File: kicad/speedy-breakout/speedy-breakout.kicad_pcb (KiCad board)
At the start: 2 copper layers, 100 x 50 mm, 7 parts, among them J1 Pin Socket 1x20, J2 Pin Socket 1x20, J3 Molex Mini-Lock 53426, J4 Molex Mini-Lock 53426, J5 CUI TLB009-254, J6 CUI TBL009-254

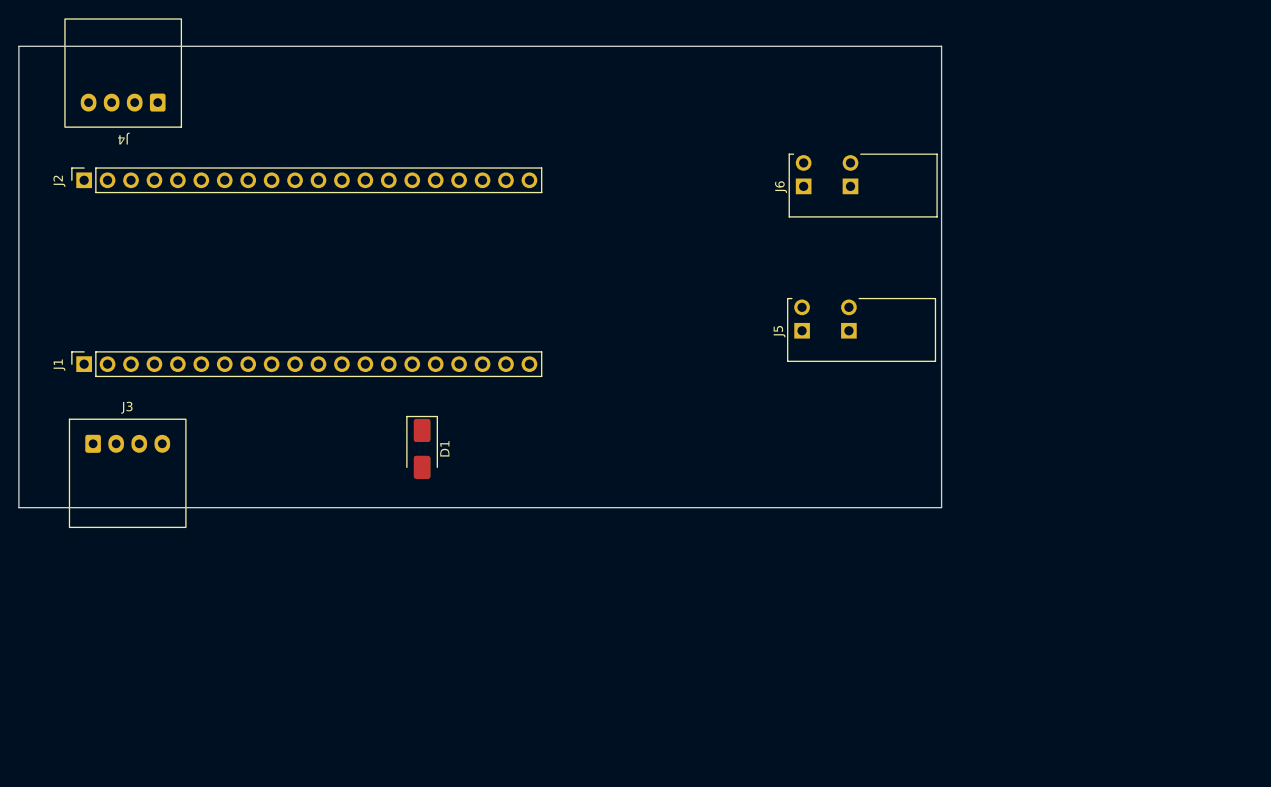
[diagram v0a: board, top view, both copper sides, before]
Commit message: speedy-breakout: Complete Rev 1.0 Schematics/Layout
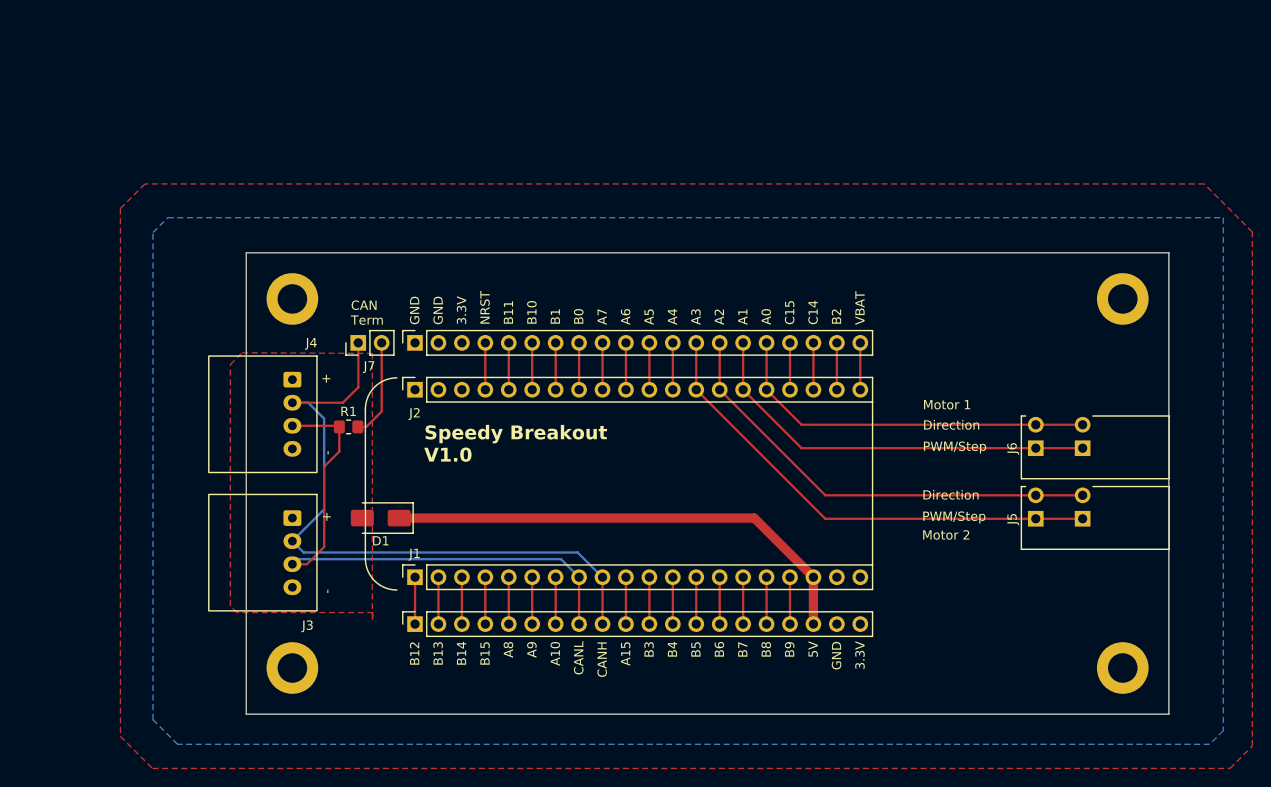
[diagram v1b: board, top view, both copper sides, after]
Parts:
- added ?: Pin Socket 1x20, Connector_PinSocket_2.54mm:PinSocket_1x20_P2.54mm_Vertical, F.Cu at (118.3, 84.8)
- added ?: Pin Socket 1x20, Connector_PinSocket_2.54mm:PinSocket_1x20_P2.54mm_Vertical, F.Cu at (118.3, 115.2)
- added J7: Conn_01x02, Connector_PinHeader_2.54mm:PinHeader_1x02_P2.54mm_Vertical, F.Cu at (112.1, 84.8)
- added R1: 120, Resistor_SMD:R_0805_2012Metric_Pad1.20x1.40mm_HandSolder, F.Cu at (111.1, 93.9)
- added REF**: MountingHole_3.2mm_M3_DIN965_Pad, MountingHole:MountingHole_3.2mm_M3_DIN965_Pad, F.Cu at (195.0, 80.0)
- added REF**: MountingHole_3.2mm_M3_DIN965_Pad, MountingHole:MountingHole_3.2mm_M3_DIN965_Pad, F.Cu at (105.0, 120.0)
- added REF**: MountingHole_3.2mm_M3_DIN965_Pad, MountingHole:MountingHole_3.2mm_M3_DIN965_Pad, F.Cu at (195.0, 120.0)
- added REF**: MountingHole_3.2mm_M3_DIN965_Pad, MountingHole:MountingHole_3.2mm_M3_DIN965_Pad, F.Cu at (105.0, 80.0)
- moved J1 42.7 mm to (118.3, 110.2)
- moved J2 42.4 mm to (118.3, 89.8)
- moved J6 37.9 mm to (185.6, 96.2)
- moved J4 33.4 mm to (105.0, 88.8), turned to -90 degrees
- moved J5 32.5 mm to (185.6, 103.8)
- moved J3 23.1 mm to (105.0, 103.8), turned to -90 degrees
- moved D1 8.74 mm to (114.6, 103.8), turned to 180 degrees
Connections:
- J2 pad 17: unconnected-(J2-Pin_17-Pad17) -> /OSC32_OUT
- J2 pad 18: unconnected-(J2-Pin_18-Pad18) -> /OSC32_IN
- J5 pad 1: unconnected-(J5-Pin_1-Pad1) -> /PA3
- J5 pad 2: unconnected-(J5-Pin_2-Pad2) -> /PA2
- J6 pad 1: unconnected-(J6-Pin_1-Pad1) -> /PA1
- J6 pad 2: unconnected-(J6-Pin_2-Pad2) -> /PA0
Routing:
- net /CANH: track 0.00 -> 71.8 mm
- net /CANL: track 0.00 -> 60.2 mm
- net /PA3: track 0.00 -> 52.8 mm
- net +5V: track 0.00 -> 52.6 mm
- net /PA2: track 0.00 -> 49.2 mm
- net /PA1: track 0.00 -> 44.5 mm
- net /PA0: track 0.00 -> 40.9 mm
- net Net-(J7-Pin_2): track 0.00 -> 10.7 mm
- net /PB9: track 0.00 -> 5.08 mm
- net /PB8: track 0.00 -> 5.08 mm
- net /PB7: track 0.00 -> 5.08 mm
- net /PB6: track 0.00 -> 5.08 mm
- net /PB5: track 0.00 -> 5.08 mm
- net /PB4: track 0.00 -> 5.08 mm
- net /PB3: track 0.00 -> 5.08 mm
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- added copper zone on F.Cu, net +3.3V
- added copper zone on B.Cu, net GND
- added copper zone on F.Cu, net Net-(D1-A)
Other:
- board text added: "+"
- board text added: "-"
- board text added: "3.3V"
- board text added: "5V"
- board text added: "A0"
- board text added: "A1"
- board text added: "A10"
- board text added: "A15"
- board text added: "A2"
- board text added: "A3"
- board text added: "A4"
- board text added: "A5"
- board text added: "A6"
- board text added: "A7"
- board text added: "A8"
- board text added: "A9"
- board text added: "B0"
- board text added: "B1"
- board text added: "B10"
- board text added: "B11"
- board text added: "B12"
- board text added: "B13"
- board text added: "B14"
- board text added: "B15"
- board text added: "B2"
- board text added: "B3"
- board text added: "B4"
- board text added: "B5"
- board text added: "B6"
- board text added: "B7"
- board text added: "B8"
- board text added: "B9"
- board text added: "C14"
- board text added: "C15"
- board text added: "CAN Term"
- board text added: "CANH"
- board text added: "CANL"
- board text added: "Direction"
- board text added: "GND"
- board text added: "Motor 1"
- board text added: "Motor 2"
- board text added: "NRST"
- board text added: "PWM/Step"
- board text added: "Speedy Breakout V1.0"
- board text added: "VBAT"
